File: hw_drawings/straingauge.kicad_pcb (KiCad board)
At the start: 4 copper layers, 130.3 x 73.4 mm, 174 parts, among them J1 Conn_01x10_Pin, J2 Conn_01x08_Pin, J3 Conn_01x08_Pin, J4 Pin, J5 Pin, U1 AD7124-8BCPZ, U10 LT3045xDD, U11 LT3045xDD, U2 LT8333RDD-PBF, U4 LT3094xDD, U5 LT8333RDD-PBF, U6 Pico, U7 SI8380PM-IU, U9 SIT8008BC-83-33E-2.4576

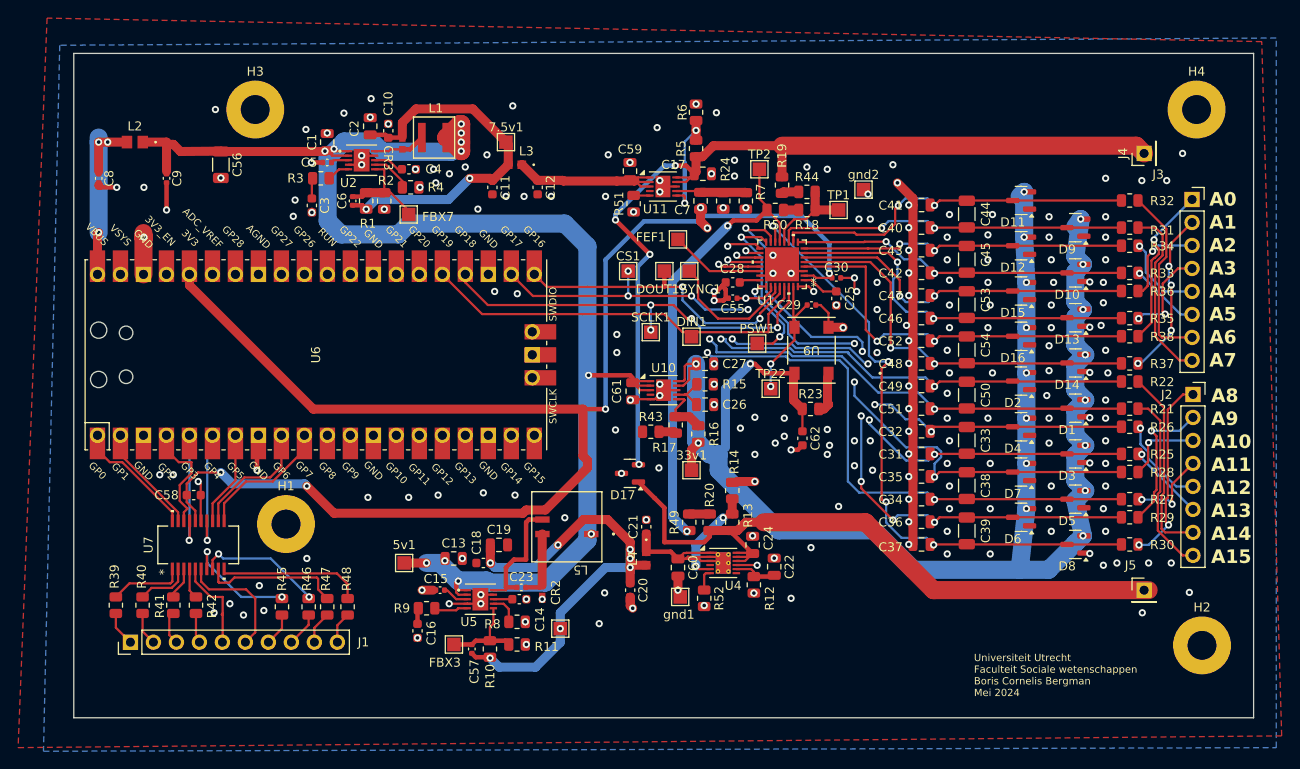
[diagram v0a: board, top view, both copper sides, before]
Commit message: changed bead
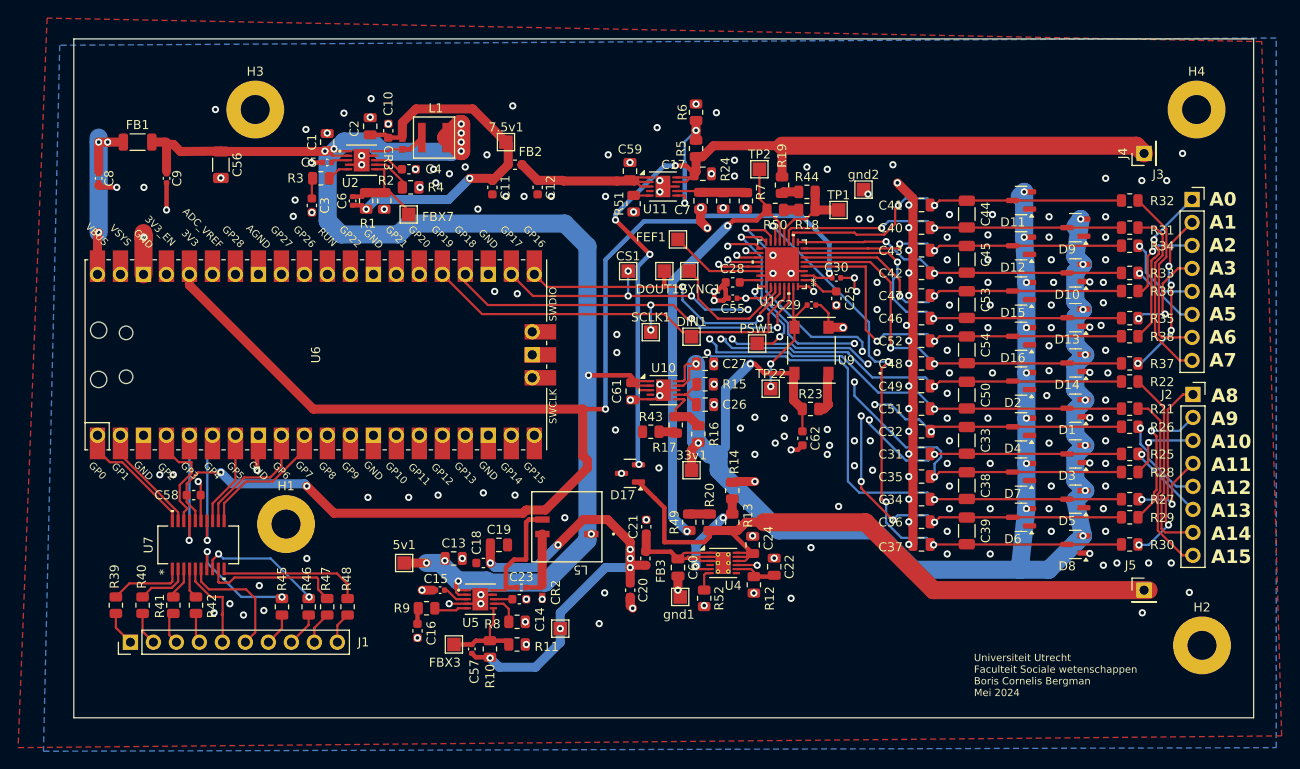
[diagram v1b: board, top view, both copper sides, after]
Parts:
- removed L2: 742792040, ul_7429:IND_742792040_WRE
- removed L3, L4: NFZ18SM121SN10D, NFZ18SM121SN10D:IND_NFZ18SM121SN10D_MUR
- added FB1: 500 2A, Inductor_SMD:L_1206_3216Metric, F.Cu at (95.8, 39.0)
- added FB2: 120 1A, Inductor_SMD:L_0603_1608Metric, F.Cu at (137.5, 41.5)
- added FB3: 120 1A, Inductor_SMD:L_0603_1608Metric, F.Cu at (151.9, 85.0)
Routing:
- net +5V: track 165.4 -> 164.5 mm
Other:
- board size 130.3 x 73.4 mm -> 130.3 x 75 mm
